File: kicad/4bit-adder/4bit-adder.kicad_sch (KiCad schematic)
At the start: 13 parts, among them K1 SR11-5V-200-2C, K2 SR11-5V-200-2C, K3 SR11-5V-200-2C, SW1 A, SW2 B

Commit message: wip schema
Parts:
- removed D1: A1 Yellow, LED_THT:LED_D5.0mm, symbol Device:LED
- removed D3: Carry1 Blue, LED_THT:LED_D5.0mm, symbol Device:LED
- removed D4: Sum1 Red, LED_THT:LED_D5.0mm, symbol Device:LED
- removed K1, K2, K3: SR11-5V-200-2C, SR11_5V_200_2C:RELAY_SR11-5V-200-2C, symbol SR11-5V-200-2C:SR11-5V-200-2C
- removed R1, R3, R4: 470, Resistor_THT:R_Axial_DIN0207_L6.3mm_D2.5mm_P10.16mm_Horizontal, symbol Device:R
- removed SW1: A, Button_Switch_THT:SW_DIP_SPSTx04_Piano_10.8x11.72mm_W7.62mm_P2.54mm, symbol Switch:SW_DIP_x04
- removed SW2: B, Button_Switch_THT:SW_DIP_SPSTx04_Piano_10.8x11.72mm_W7.62mm_P2.54mm, symbol Switch:SW_DIP_x04
- added D1, D3, D4: 1N4007, Diode_THT:D_DO-41_SOD81_P10.16mm_Horizontal, symbol Diode:1N4007
- added D10: A4 Yellow, LED_THT:LED_D5.0mm, symbol Device:LED
- added D11: Carry2 White, LED_THT:LED_D5.0mm, symbol Device:LED
- added D12: Carry3 White, LED_THT:LED_D5.0mm, symbol Device:LED
- added D15: B4 Green, LED_THT:LED_D5.0mm, symbol Device:LED
- added D16: A3 Yellow, LED_THT:LED_D5.0mm, symbol Device:LED
- added D17: B3 Green, LED_THT:LED_D5.0mm, symbol Device:LED
- added D18: A2 Yellow, LED_THT:LED_D5.0mm, symbol Device:LED
- added D19: B2 Green, LED_THT:LED_D5.0mm, symbol Device:LED
- added D21: B1 Green, LED_THT:LED_D5.0mm, symbol Device:LED
- added D8: Sum1 Red, LED_THT:LED_D5.0mm, symbol Device:LED
- added D9: Carry1 White, LED_THT:LED_D5.0mm, symbol Device:LED
- added J1: Screw_Terminal_01x02, TerminalBlock:TerminalBlock_MaiXu_MX126-5.0-02P_1x02_P5.00mm, symbol Connector:Screw_Terminal_01x02
- added K1, K10, K11, K12, K13, K14, K15, K17, K18, K2, K3, K4, K5, K6: SR11-5V-200-2C-PH, SR11_5V_200_2C:RELAY_SR11-5V-200-2C, symbol SR11-5V-200-2C:SR11-5V-200-2C-PH
- added K7, K8, K9: SR11-5V-200-2C, SR11_5V_200_2C:RELAY_SR11-5V-200-2C, symbol SR11-5V-200-2C:SR11-5V-200-2C
- added R10, R15, R16, R17, R18, R19, R20, R21, R22, R23, R8: 470, Resistor_THT:R_Axial_DIN0207_L6.3mm_D2.5mm_P10.16mm_Horizontal, symbol Device:R
- added SW3: A, Button_Switch_THT:SW_DIP_SPSTx04_Piano_10.8x11.72mm_W7.62mm_P2.54mm, symbol Switch:SW_DIP_x04
- added SW4: B, Button_Switch_THT:SW_DIP_SPSTx04_Piano_10.8x11.72mm_W7.62mm_P2.54mm, symbol Switch:SW_DIP_x04
- D2: value B1 Green -> A1 Yellow
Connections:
- net +5V: now also J1.1 (Pin_1), K4.COM2, K6.COM2, K9.COM2, SW3.5, SW3.6, SW3.7, SW3.8, SW4.5, SW4.6, SW4.7, SW4.8
- net GND: now also J1.2 (Pin_2), K1.A1, K17.A1, K2.A1, K3.A1, K4.A1, K6.A1, K7.A1, K8.A1, K9.A1, R10.2, R15.2, R16.2, R17.2, R18.2, R19.2, R20.2, R21.2, R22.2, R23.2, R8.2
- net at D2.2 (A): now also K7.COM1, K8.A2, SW3.1
- new net: D19.1 (K), R19.1
- new net: D19.2 (A), K5.A2, SW4.2
- new net: D12.1 (K), R23.1
- new net: D8.1 (K), R8.1
- new net: D8.2 (A), K8.COM2
- new net: D15.1 (K), R15.1
- new net: D21.2 (A), K7.A2, K9.A2, SW4.1
- new net: D17.2 (A), SW4.3
- new net: K8.NO2, K9.NC2
- new net: K8.NC2, K9.NO2
- new net: D9.2 (A), K17.A2, K7.NC1
- new net: K5.A1, K6.A2
- new net: K4.NO2, K5.NC2
- new net: K4.NC2, K5.NO2
- new net: D11.1 (K), R22.1
- new net: D18.2 (A), K1.COM1, K2.COM1, K4.A2, SW3.2
- new net: D3.2 (A), K2.NO1
- new net: D9.1 (K), R20.1
- new net: D17.1 (K), R17.1
- new net: D10.1 (K), R10.1
- new net: D1.2 (A), K1.NO1
- new net: D16.1 (K), R16.1
- new net: K17.NC2, K6.NO2
- new net: K17.NO2, K6.NC2
- new net: D21.1 (K), R21.1
- new net: D4.2 (A), K3.NO1
- new net: D18.1 (K), R18.1
- new net: D16.2 (A), SW3.3
- no-connect marks 10 -> 30

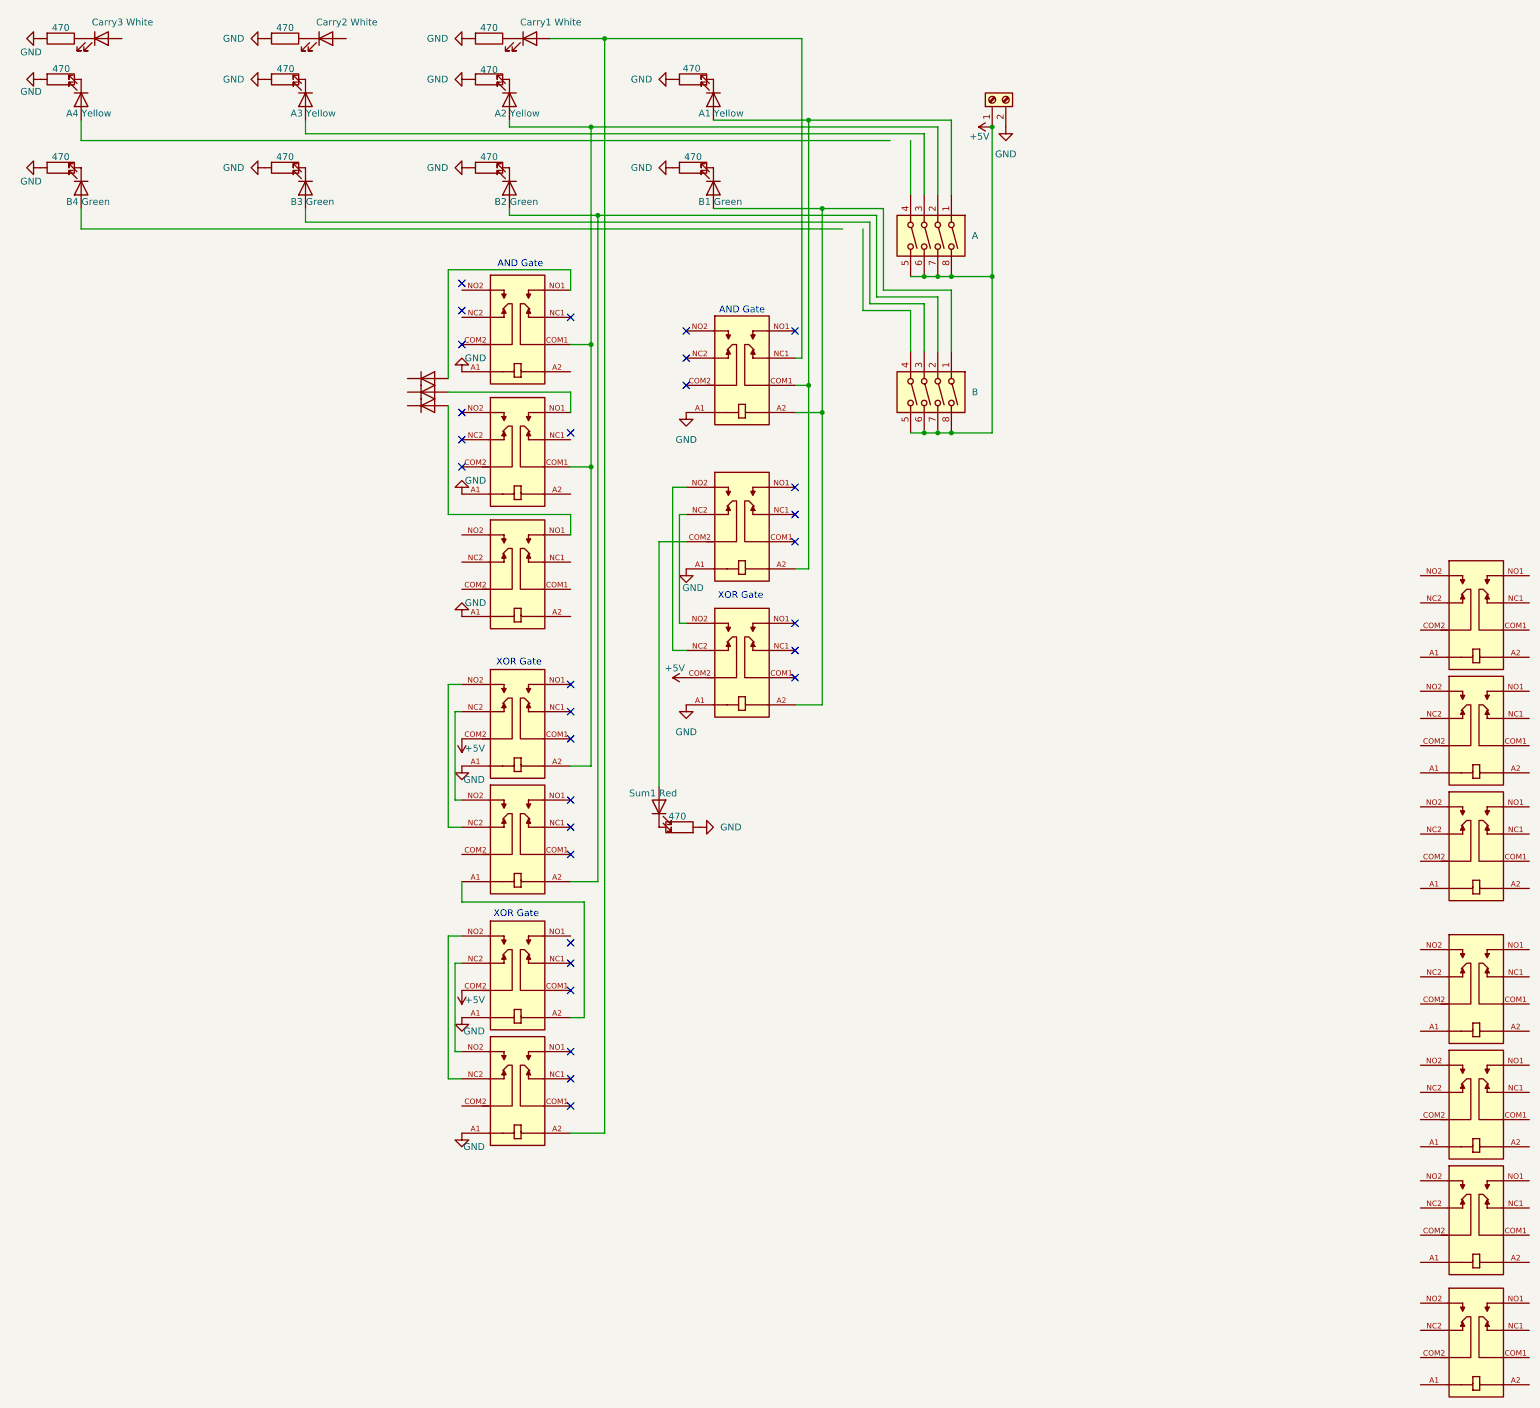
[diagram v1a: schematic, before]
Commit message: schematic first draft
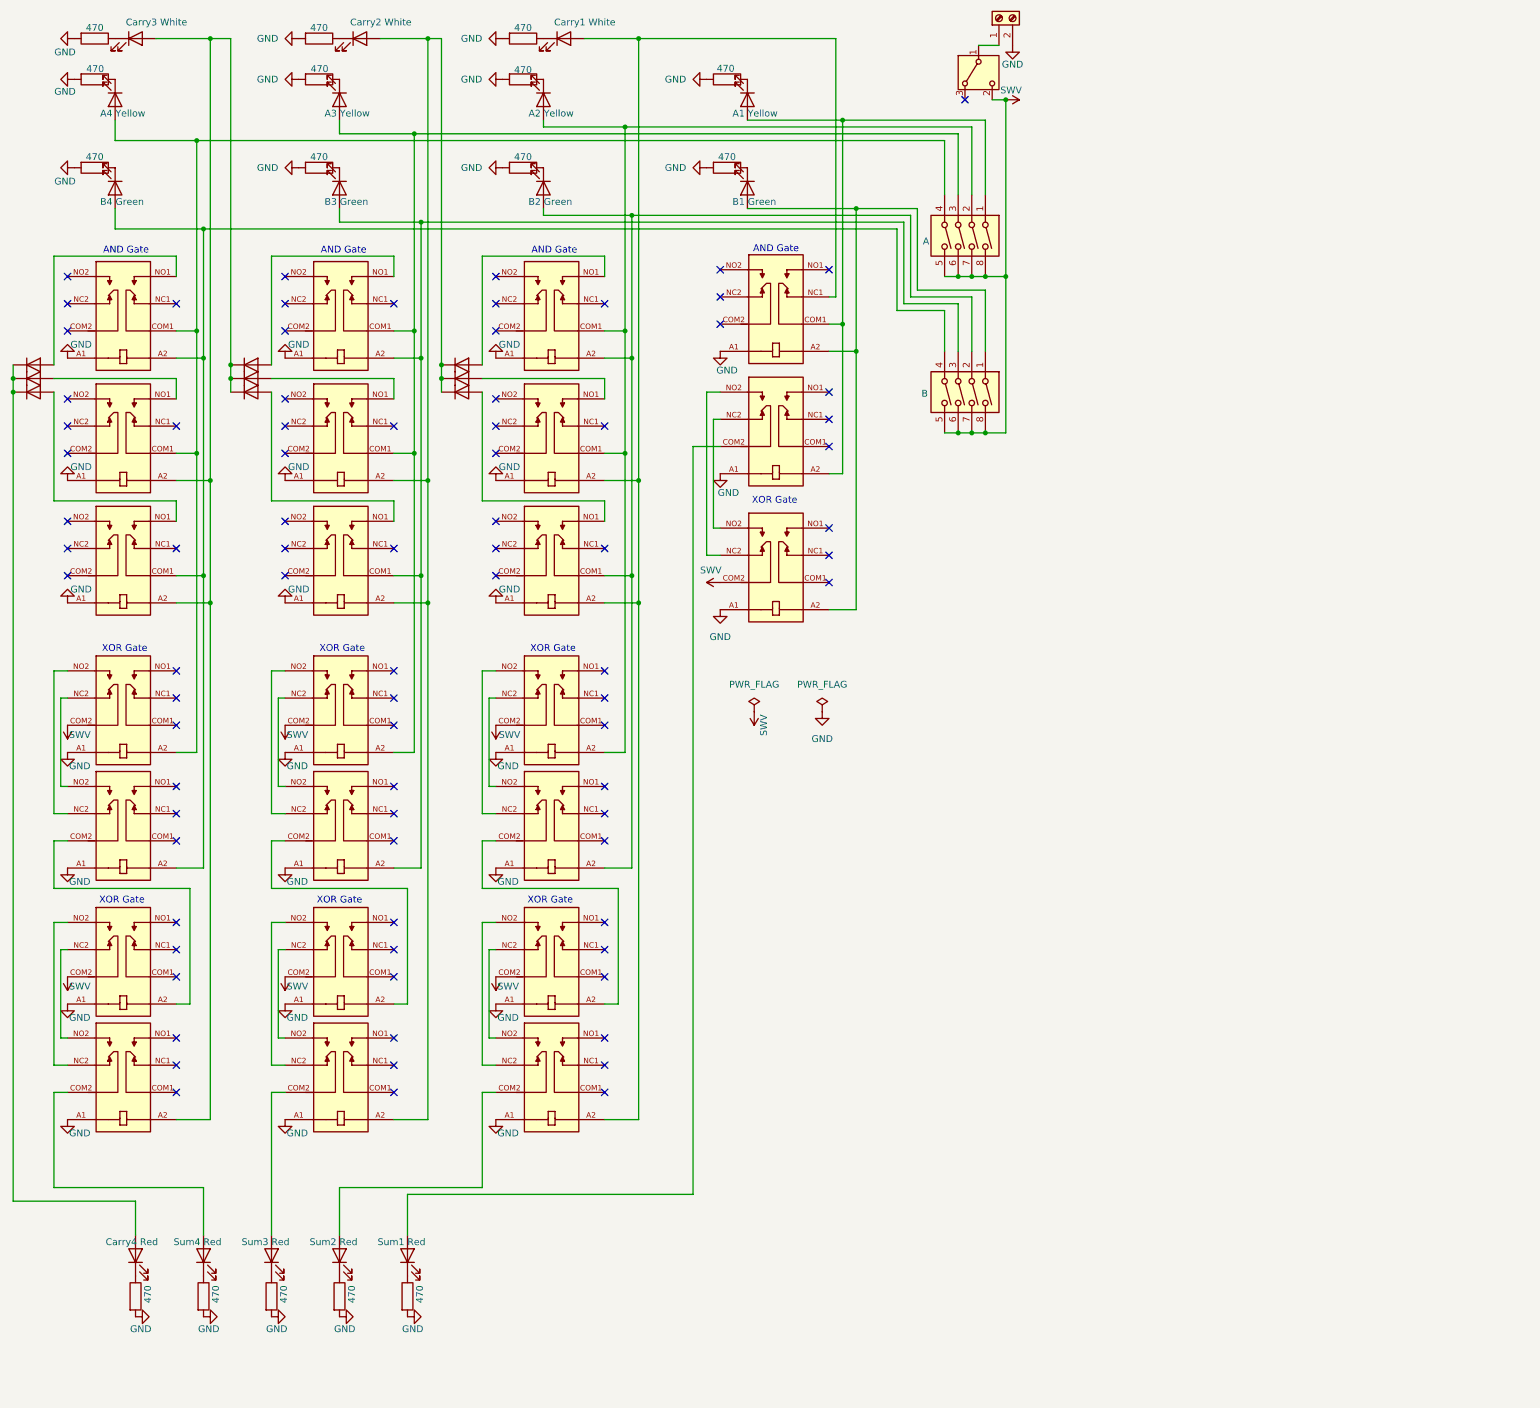
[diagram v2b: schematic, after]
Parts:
- removed K7, K8, K9: SR11-5V-200-2C, SR11_5V_200_2C:RELAY_SR11-5V-200-2C, symbol SR11-5V-200-2C:SR11-5V-200-2C
- added D13: Sum2 Red, LED_THT:LED_D5.0mm, symbol Device:LED
- added D14: Sum3 Red, LED_THT:LED_D5.0mm, symbol Device:LED
- added D20: Sum4 Red, LED_THT:LED_D5.0mm, symbol Device:LED
- added D22, D23, D24, D5, D6, D7: 1N4007, Diode_THT:D_DO-41_SOD81_P10.16mm_Horizontal, symbol Diode:1N4007
- added D25: Carry4 Red, LED_THT:LED_D5.0mm, symbol Device:LED
- added K16, K19, K20, K21, K22, K23, K24, K7, K8, K9: SR11-5V-200-2C-PH, SR11_5V_200_2C:RELAY_SR11-5V-200-2C, symbol SR11-5V-200-2C:SR11-5V-200-2C-PH
- added R11, R12, R13, R9: 470, Resistor_THT:R_Axial_DIN0207_L6.3mm_D2.5mm_P10.16mm_Horizontal, symbol Device:R
- added SW1: SW_Wuerth_450301014042, Button_Switch_THT:SW_Slide-03_Wuerth-WS-SLTV_10x2.5x6.4_P2.54mm, symbol Switch:SW_Wuerth_450301014042
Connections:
- net GND: now also K10.A1, K11.A1, K12.A1, K13.A1, K14.A1, K15.A1, K18.A1, K5.A1, K16.A1, K19.A1, K20.A1, K21.A1, K22.A1, K23.A1, K24.A1, K7.A1, K8.A1, K9.A1, R11.2, R12.2, R13.2, R9.2
- net at K18.A2: now also D1.1 (K), D11.2 (A), D3.1 (K), D4.1 (K), K11.A2, K12.A2
- net at K18.COM2: now also D14.2 (A)
- net at K18.NC2: now also K15.NO2
- net at K18.NO2: now also K15.NC2
- net at K10.A2: now also D17.2 (A), K12.COM1, K14.A2, SW4.3
- net at K10.COM1: now also D16.2 (A), K11.COM1, K13.A2, SW3.3
- net at K10.NO1: now also D5.2 (A)
- net at D19.2 (A), K5.A2, SW4.2: now also K1.A2, K3.COM1
- net at D12.2 (A): now also D5.1 (K), D6.1 (K), D7.1 (K), K19.A2, K20.A2, K24.A2
- net at D8.2 (A): now also K8.COM2
- net at D15.2 (A): now also SW4.4, K16.A2, K20.COM1, K22.A2
- net at K11.NO1: now also D6.2 (A)
- net at K15.A2: now also K14.COM2
- net SWV: now reaches K15.COM2
- net SWV: now also K13.COM2, K4.COM2, K6.COM2, SW3.5, SW3.6, SW3.7, SW3.8, SW4.5, SW4.6, SW4.7, SW4.8, K21.COM2, K23.COM2, K9.COM2, SW1.2 (C)
- net at D21.2 (A), SW4.1: now also K7.A2, K9.A2
- net at D2.2 (A), SW3.1: now also K7.COM1, K8.A2
- net at D9.2 (A), K17.A2: now also K2.A2, K3.A2, K7.NC1
- net at K6.A2: now also K5.COM2; no longer K5.A1
- net at K14.NC2: now also K13.NO2
- net at K14.NO2: now also K13.NC2
- net at D10.2 (A): now also SW3.4, K16.COM1, K19.COM1, K21.A2
- net at K17.COM2: now also D13.2 (A)
- net at K12.NO1: now also D7.2 (A)
- removed net +5V: J1.1 (Pin_1), K4.COM2, K6.COM2, SW3.5, SW3.6, SW3.7, SW3.8, SW4.5, SW4.6, SW4.7, SW4.8
- new net: D24.2 (A), K20.NO1
- new net: K21.NC2, K22.NO2
- new net: K21.NO2, K22.NC2
- new net: D14.1 (K), R11.1
- new net: J1.1 (Pin_1), SW1.1 (B)
- new net: D20.1 (K), R12.1
- new net: D20.2 (A), K24.COM2
- new net: D22.1 (K), D23.1 (K), D24.1 (K), D25.2 (A)
- new net: D22.2 (A), K16.NO1
- new net: K22.COM2, K23.A2
- new net: K23.NC2, K24.NO2
- new net: K23.NO2, K24.NC2
- new net: D13.1 (K), R9.1
- new net: D23.2 (A), K19.NO1
- new net: K8.NO2, K9.NC2
- new net: K8.NC2, K9.NO2
- new net: D25.1 (K), R13.1
- no-connect marks 30 -> 83
